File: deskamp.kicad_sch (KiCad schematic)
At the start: 29 parts, among them J1 Input 01, J2 Input 02, J3 Preamp Out, J4 Selector Switch, J5 LFE, J6 Mute, J7 Sleep, J8 Motor, J9 Power, K1 Mute, K2 Sleep, K3 TQ2-12V, K4 TQ2-12V, Q1 PN2222A, Q2 PN2222A, Q3 PN2222A, Q4 PN2222A, U1 esp32-wemos-d1-mini, U2 L9110, U3 TSR_1-2433

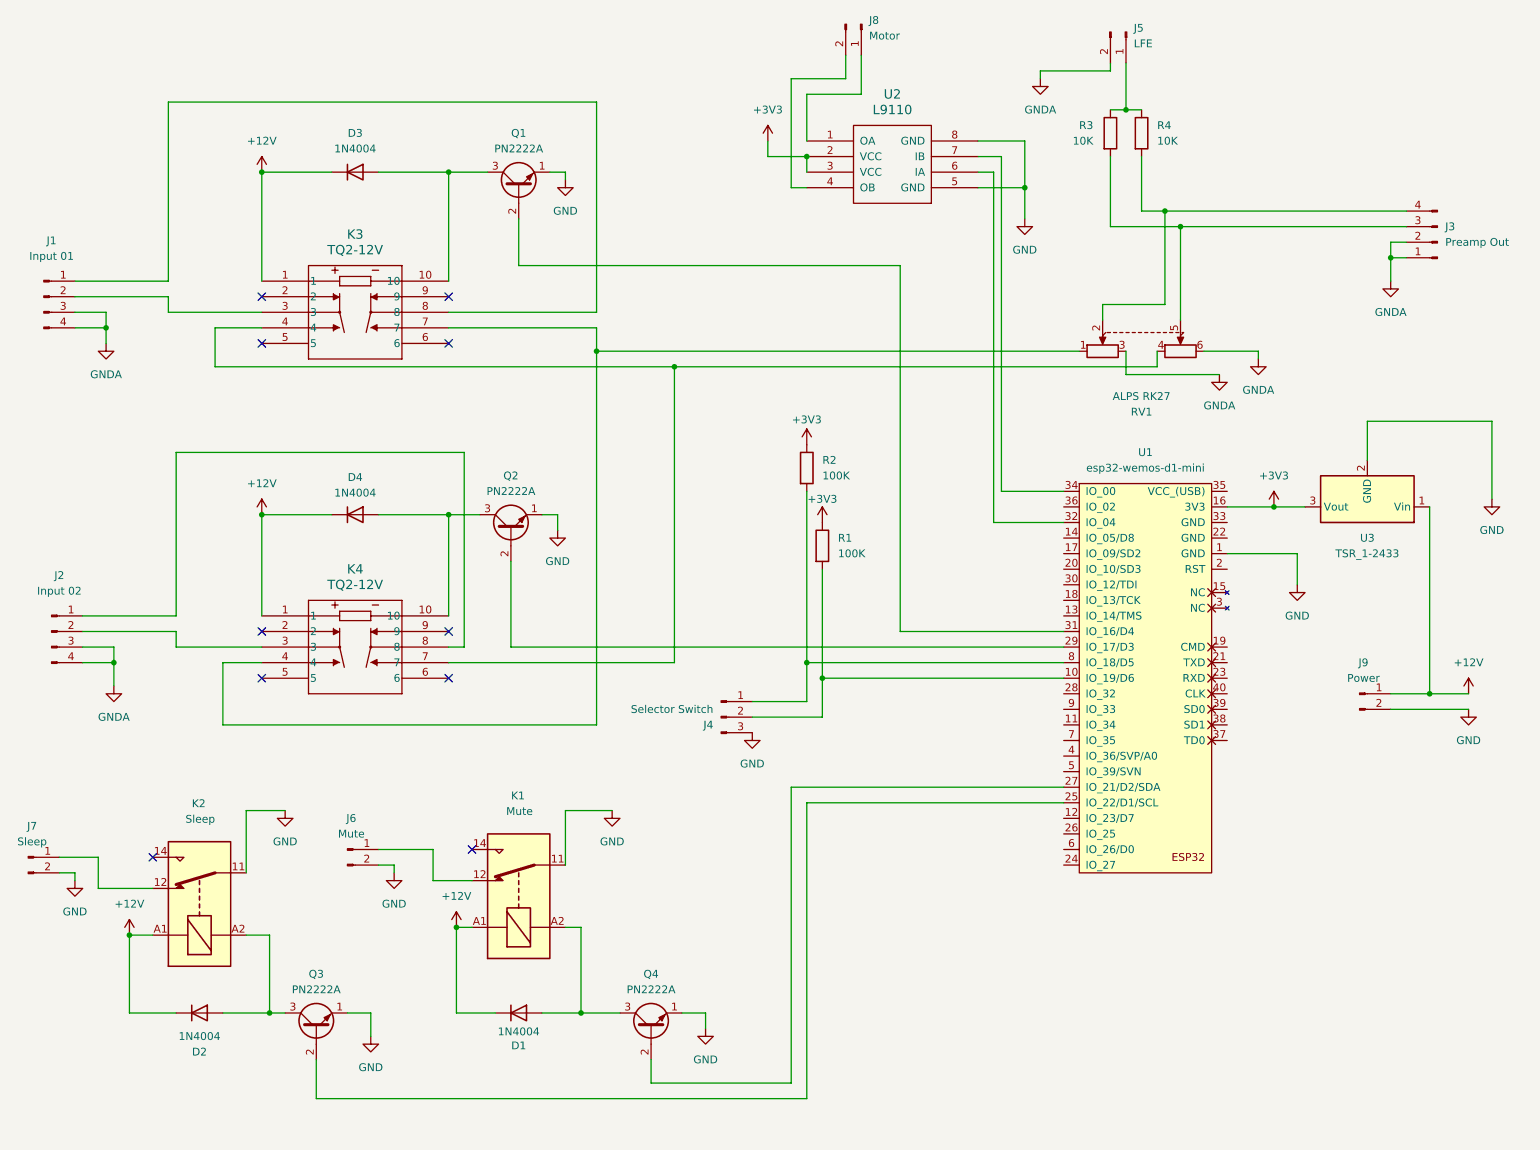
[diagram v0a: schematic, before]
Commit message: Stuck until modelling Alps pot
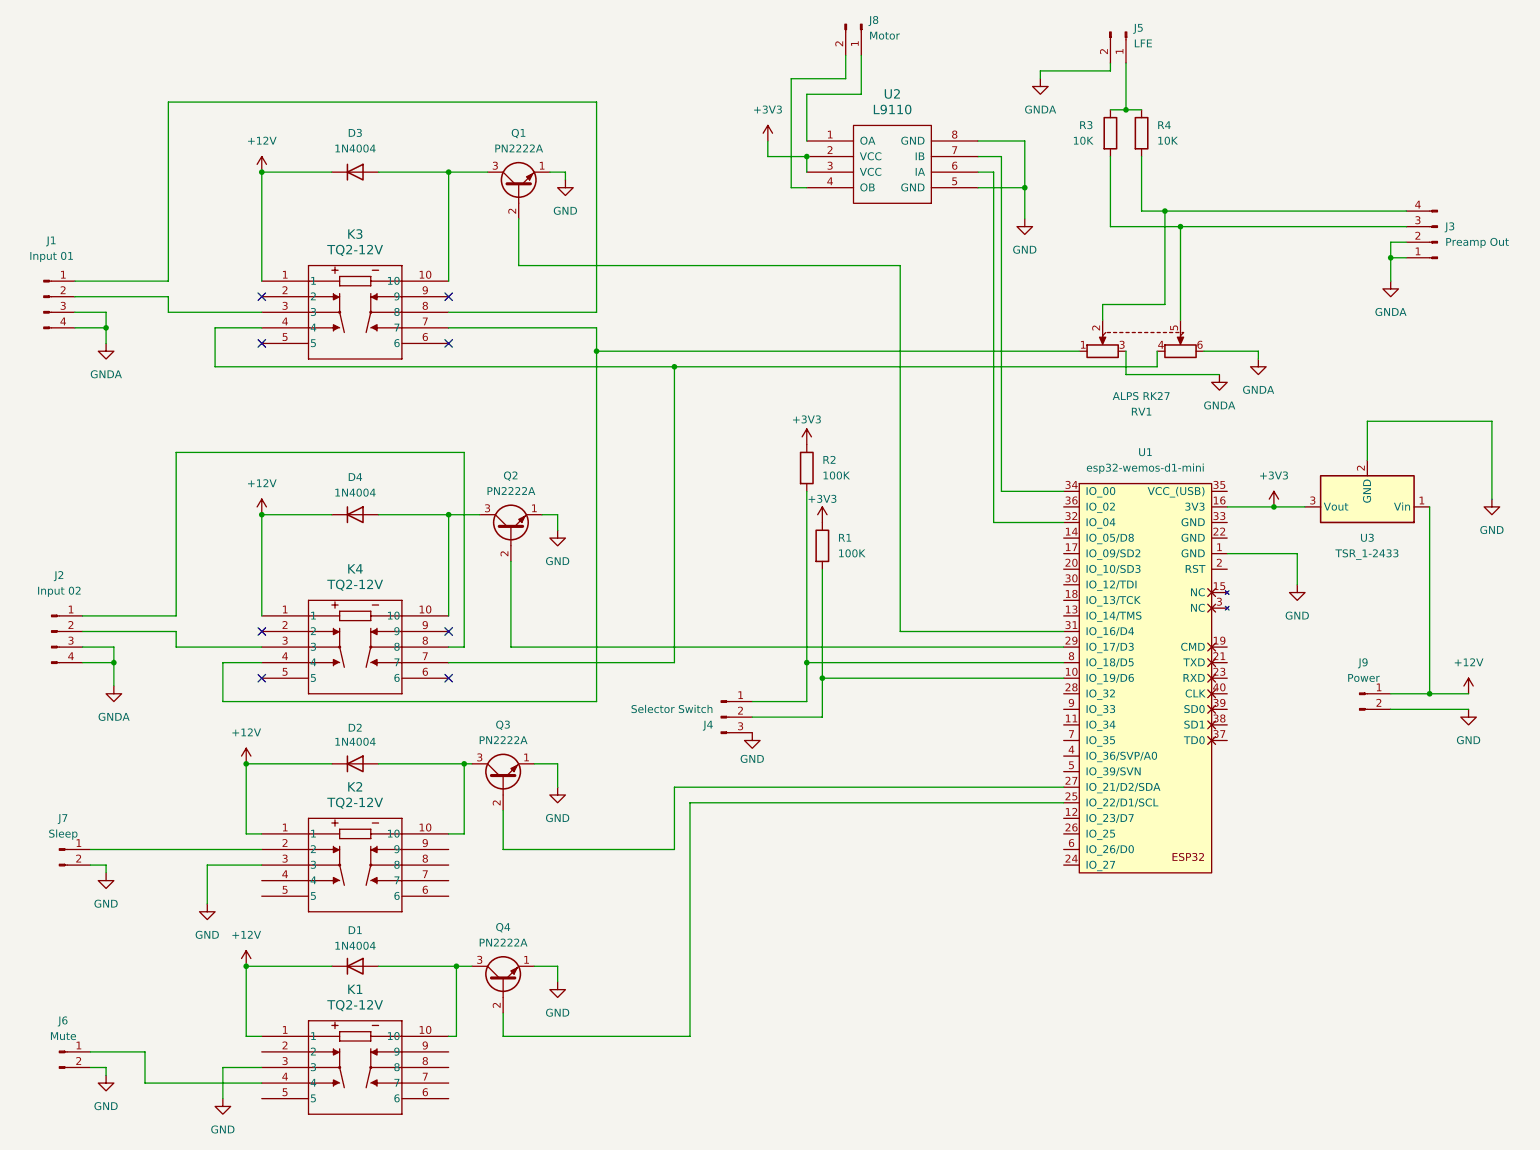
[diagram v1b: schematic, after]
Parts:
- removed K1: Mute, Relay_THT:Relay_SPDT_Panasonic_JW1_FormC, symbol Relay:Relay_SPDT
- removed K2: Sleep, Relay_THT:Relay_SPDT_Panasonic_JW1_FormC, symbol Relay:Relay_SPDT
- added K1, K2: TQ2-12V, tq2:RELAY_TQ2_PAN, symbol 2025-10-05_02-56-43:TQ2-12V
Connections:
- net +12V: now also K1.1, K2.1
- net GND: now also K1.3, K2.3
- net at Q3.2 (B): now also U1.27 (IO_21/D2/SDA); no longer U1.25 (IO_22/D1/SCL)
- net at D2.2 (A), Q3.3 (C): now also K2.10
- net at J6.1 (Pin_1): now also K1.4
- net at D1.2 (A), Q4.3 (C): now also K1.10
- net at J7.1 (Pin_1): now also K2.2
- net at Q4.2 (B): now also U1.25 (IO_22/D1/SCL); no longer U1.27 (IO_21/D2/SDA)
- no-connect marks 10 -> 8
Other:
- moved on the sheet: D1, D2, J6, J7, Q3, Q4
